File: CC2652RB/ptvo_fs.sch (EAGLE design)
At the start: 30 parts, among them IC1 DS18S20USOP8, Q1 SI2323DS, U1 SHTC3, U2 E72-2G4M05S1F, Y1 Q22FA12800150

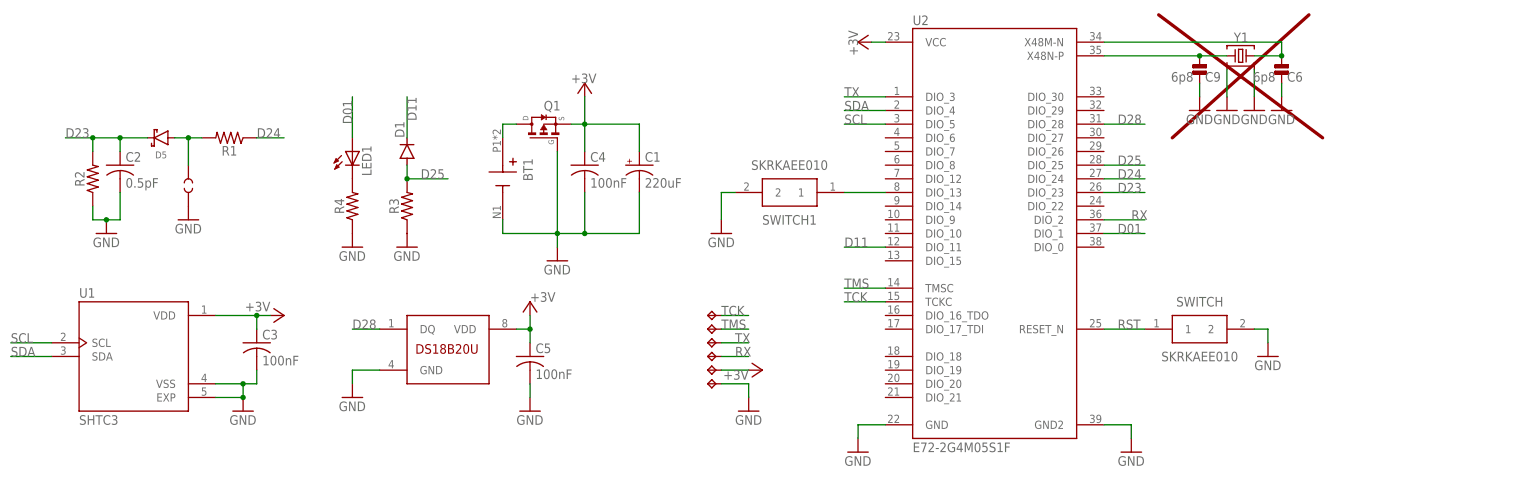
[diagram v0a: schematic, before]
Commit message: Add files via upload
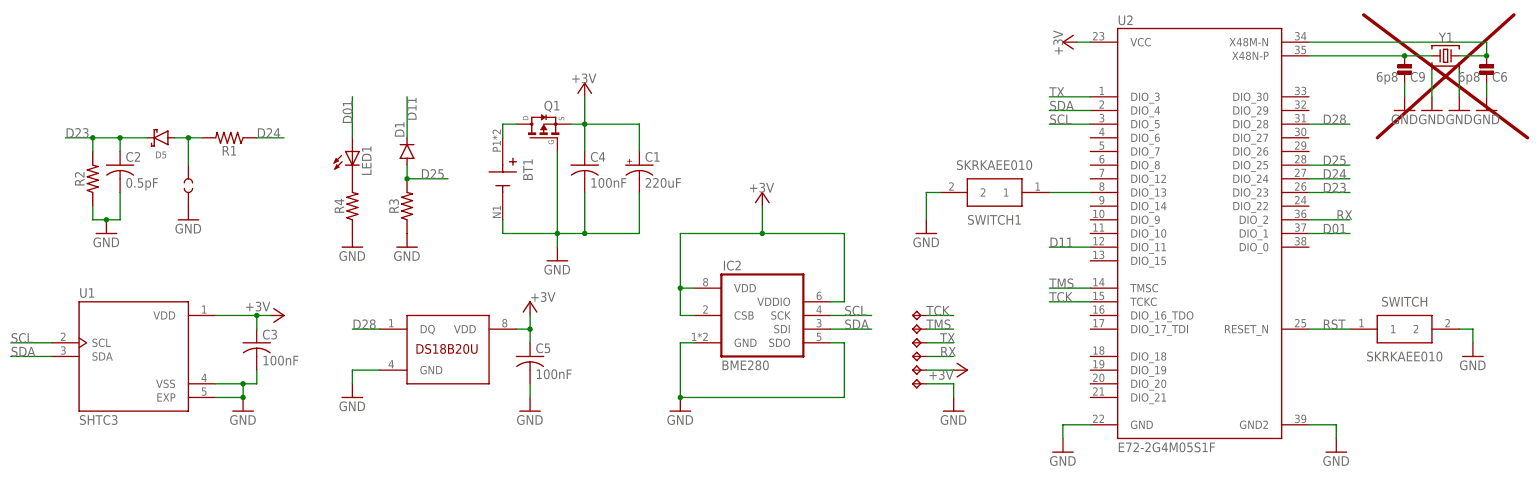
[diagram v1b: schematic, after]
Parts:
- added IC2: BME280, bosch-bme280:BME280
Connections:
- net +3V3: now also IC2.CSB, IC2.VDD, IC2.VDDIO
- net GND: now also IC2.GND, IC2.SDO
- net SCL: now also IC2.SCK
- net SDA: now also IC2.SDI
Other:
- moved on the sheet: C6, C9, SWITCH, SWITCH1, U2, Y1
